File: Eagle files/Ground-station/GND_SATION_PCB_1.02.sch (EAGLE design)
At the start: 62 parts, among them IC1 BMP280, J1 USB4110GFA, J2 XT60-M, J3 B4B-XH-AM_(LF)(SN), J6 503182-1852, U1 AMS1117-5.0, U3 AMS1117-3.3, U4 SOIC127P790X216-8NW25Q128JVJSQ

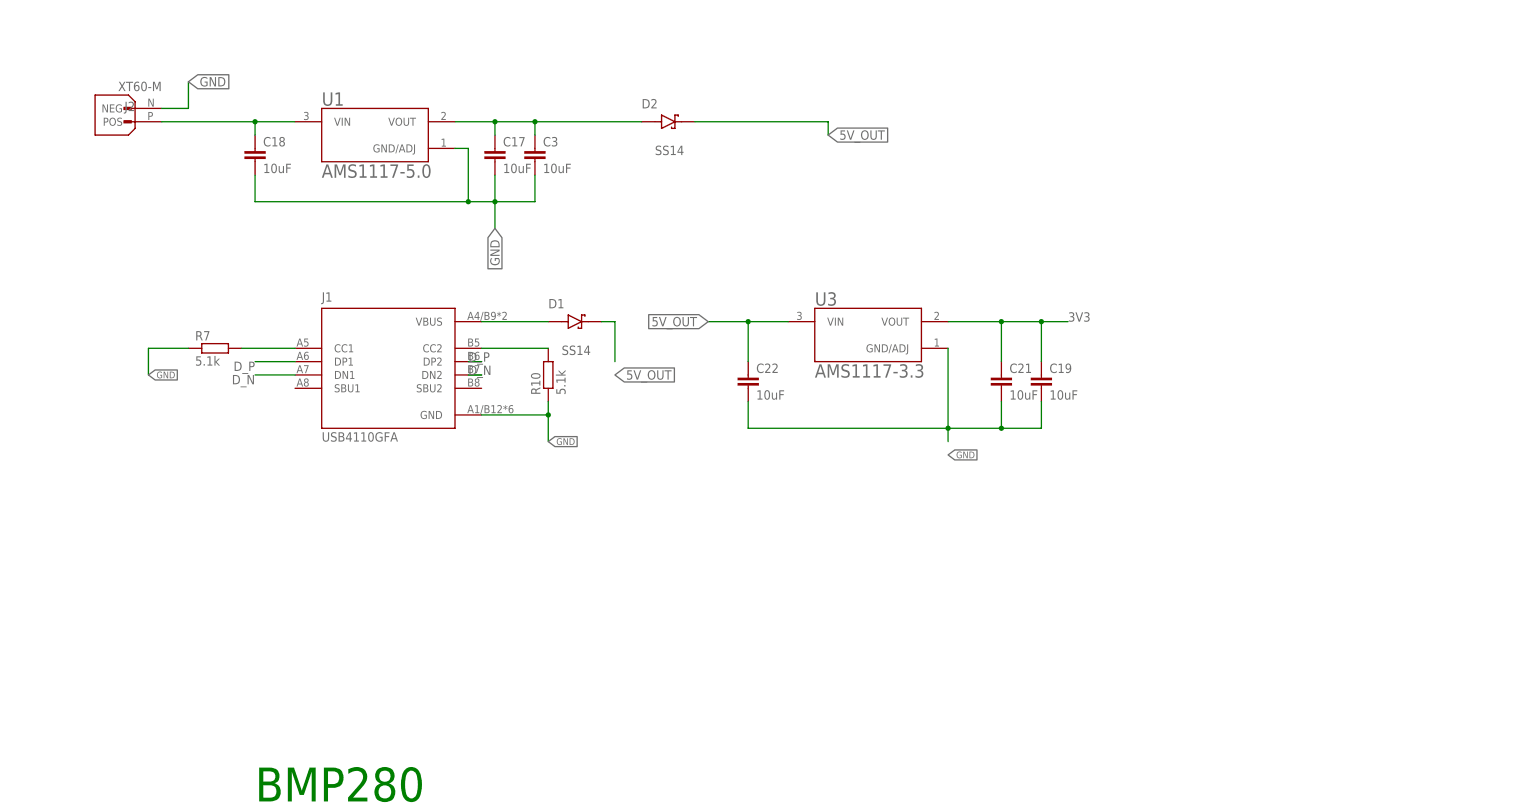
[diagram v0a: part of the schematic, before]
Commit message: pcb
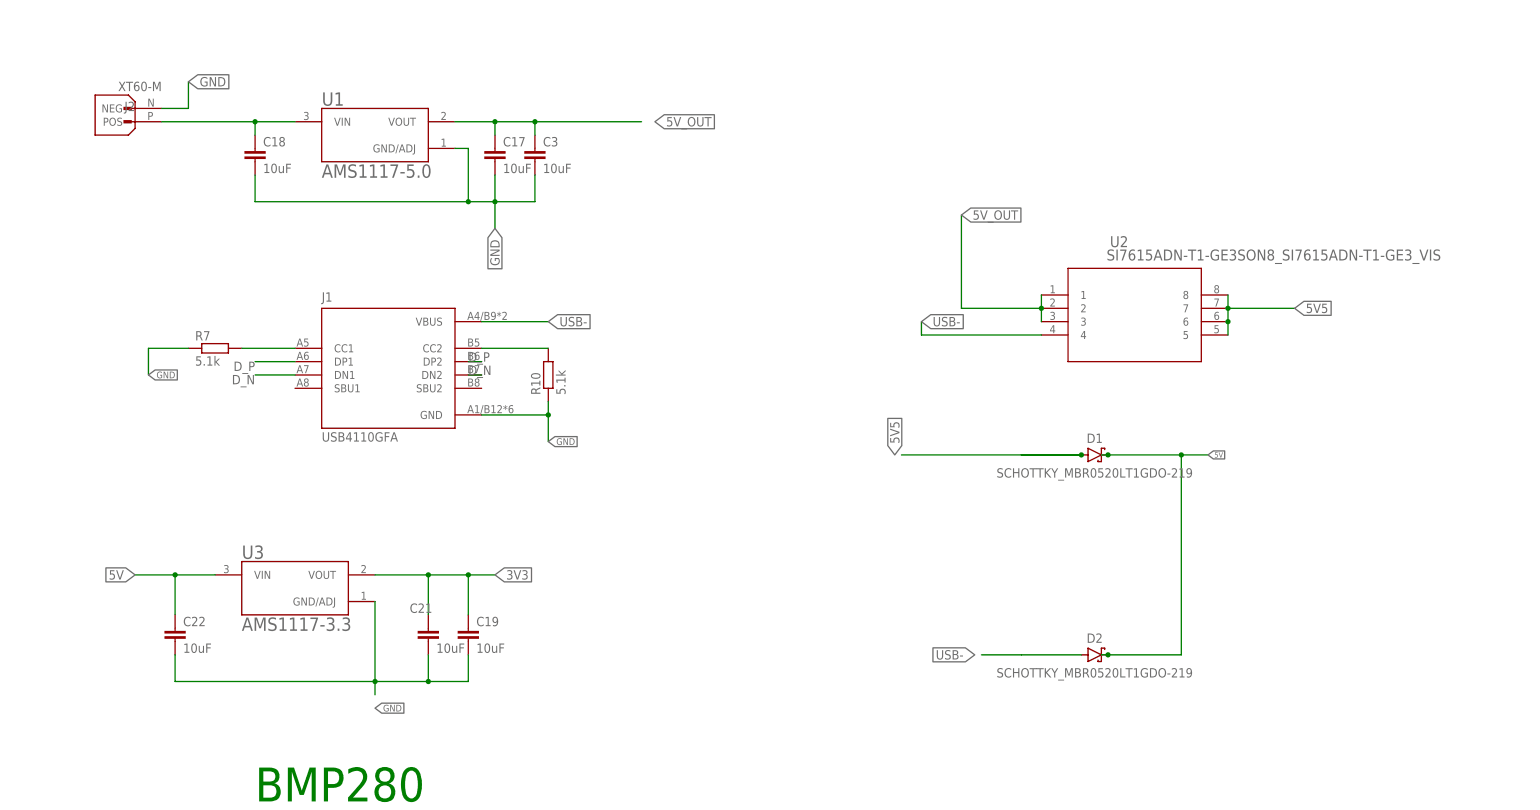
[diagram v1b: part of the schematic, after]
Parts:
- added U2: SI7615ADN-T1-GE3SON8_SI7615ADN-T1-GE3_VIS, 2025-03-10_11-27-14_Library:SI7615ADN-T1-GE3SON8_SI7615ADN-T1-GE3_VIS
- D1, D2: value SS14 -> SCHOTTKY_MBR0520LT1GDO-219; device SS14:SS14 -> Diode:SCHOTTKY_MBR0520LT1GDO-219
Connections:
- removed net N$9: D1.A, J1.VBUS
- new net 5V: C22.1, D1.C, D2.C, U3.VIN
- new net 5V5: D1.A, U2.5, U2.6, U2.7, U2.8
- new net USB-: D2.A, J1.VBUS, U2.4
- net 5V_OUT: now also U2.1, U2.2, U2.3; no longer C22.1, D1.K, D2.A, D2.K, U3.VIN
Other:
- moved on the sheet: C19, C21, C22, U3
